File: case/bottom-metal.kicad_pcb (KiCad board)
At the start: 2 copper layers, 135 x 93.7 mm, 5 parts

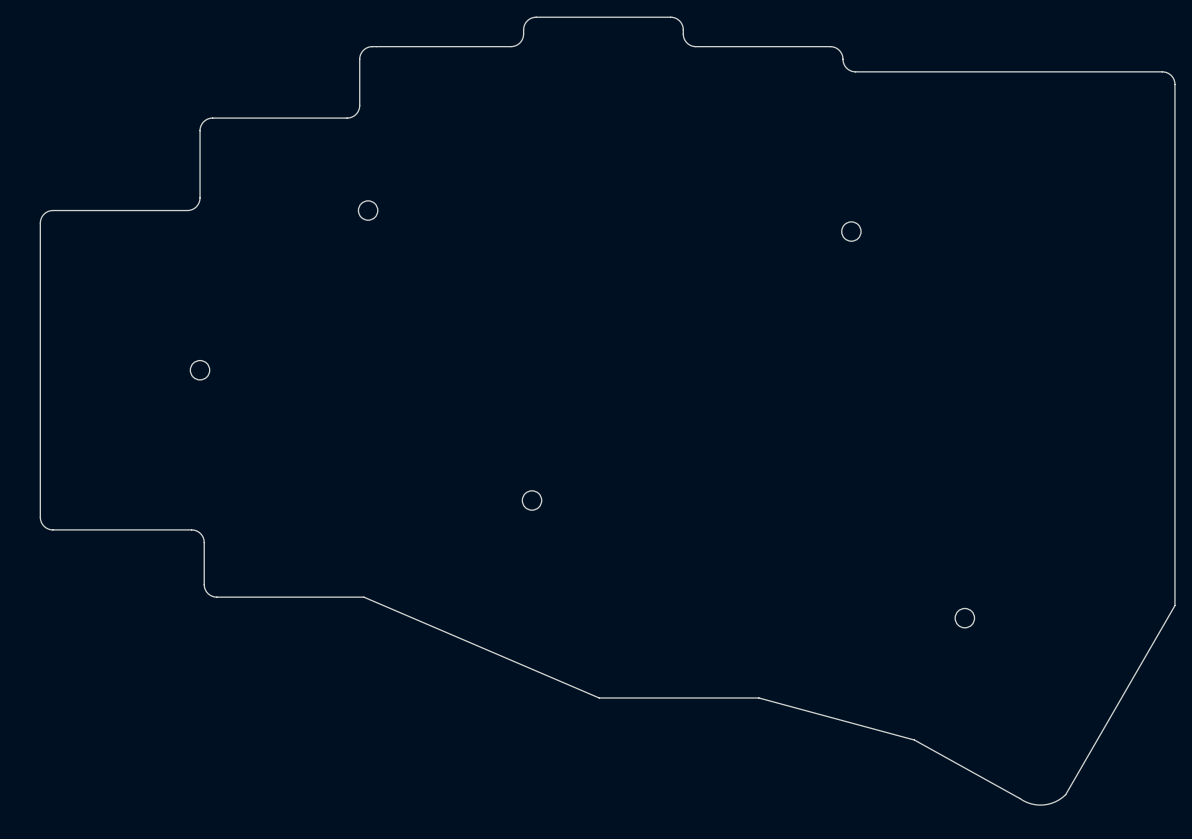
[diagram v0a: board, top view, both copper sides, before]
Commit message: update case files
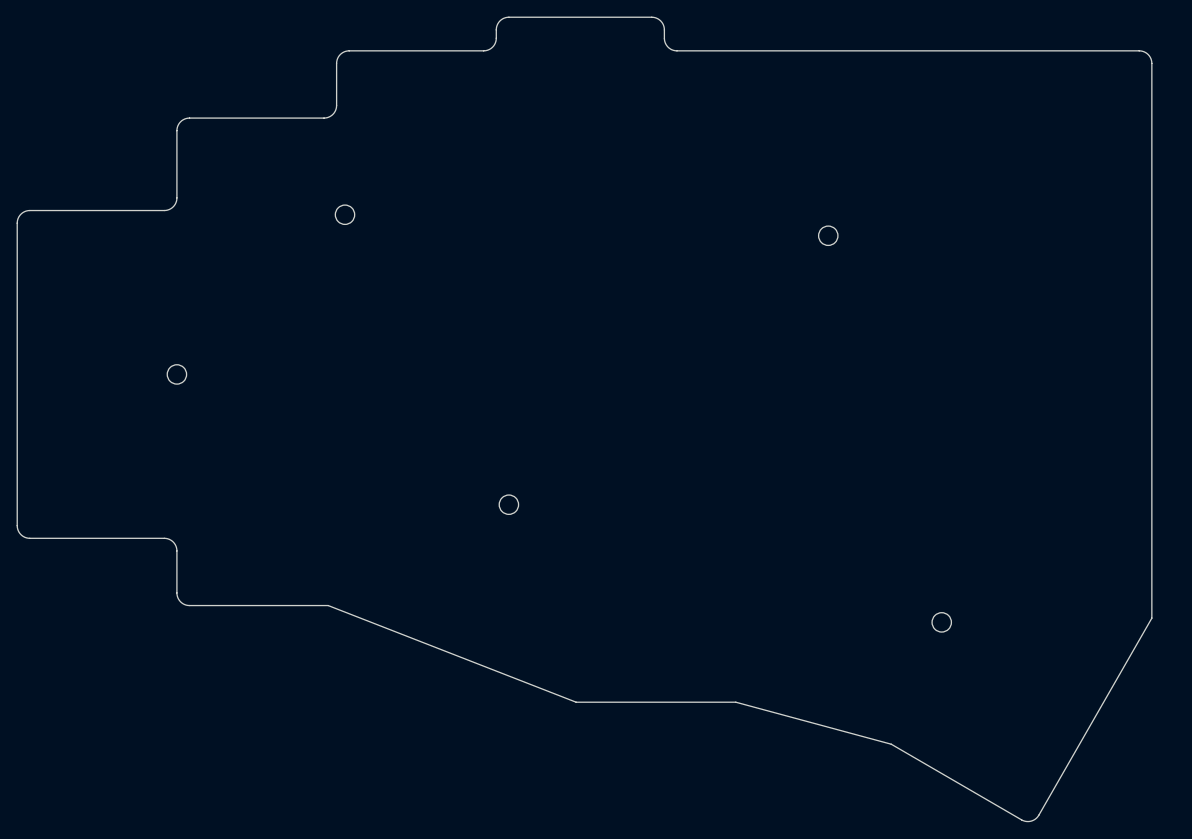
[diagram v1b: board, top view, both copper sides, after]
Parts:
- moved H1 2.80 mm to (104.8, 75.0)
- moved H2 2.80 mm to (175.8, 123.5)
- moved H3 2.80 mm to (84.8, 94.0)
- moved H4 2.80 mm to (124.2, 109.5)
- moved H5 2.80 mm to (162.2, 77.5)
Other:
- board size 135 x 93.7 mm -> 135 x 95.7 mm
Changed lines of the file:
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@@
       (drillshape 0)
       (scaleselection 1)
-      (outputdirectory "gerber/")
+      (outputdirectory "dxf/")
     )
   )
   (net 0 "")
   (footprint "kbd:thread_m2" (layer "F.Cu")
-    (at 178.5 123)
+    (at 175.75 123.5)
     (descr "Mounting Hole 2.2mm, no annular, M2")
     (tags "mounting hole 2.2mm no annular m2")
@@
   )
   (footprint "kbd:thread_m2" (layer "F.Cu")
-    (at 87.5 93.5)
+    (at 84.75 94)
     (descr "Mounting Hole 2.2mm, no annular, M2")
     (tags "mounting hole 2.2mm no annular m2")
@@
   )
   (footprint "kbd:thread_m2" (layer "F.Cu")
-    (at 165 77)
+    (at 124.25 109.5)
     (descr "Mounting Hole 2.2mm, no annular, M2")
     (tags "mounting hole 2.2mm no annular m2")
@@
     (property "Sheetname" "")
     (attr exclude_from_pos_files exclude_from_bom)
-    (fp_text reference "H5" (at -0.95 -0.55) (layer "F.Fab") hide
+    (fp_text reference "H4" (at -0.95 -0.55) (layer "F.Fab") hide
       (effects (font (size 1 1) (thickness 0.15)))
     )
@@
   )
   (footprint "kbd:thread_m2" (layer "F.Cu")
-    (at 107.5 74.5)
+    (at 104.75 75)
     (descr "Mounting Hole 2.2mm, no annular, M2")
     (tags "mounting hole 2.2mm no annular m2")
@@
   )
   (footprint "kbd:thread_m2" (layer "F.Cu")
-    (at 127 109)
+    (at 162.25 77.5)
     (descr "Mounting Hole 2.2mm, no annular, M2")
     (tags "mounting hole 2.2mm no annular m2")
@@
     (property "Sheetname" "")
     (attr exclude_from_pos_files exclude_from_bom)
-    (fp_text reference "H4" (at -0.95 -0.55) (layer "F.Fab") hide
+    (fp_text reference "H5" (at -0.95 -0.55) (layer "F.Fab") hide
       (effects (font (size 1 1) (thickness 0.15)))
     )
@@
     (pad "" np_thru_hole circle locked (at 0 0) (size 2.3 2.3) (drill 2.3) (layers *.Cu *.Mask))
   )
-  (gr_line (start 126 53) (end 126 53.5) (layer "Edge.Cuts") (width 0.1))
-  (gr_line (start 145 53.5) (end 145 53) (layer "Edge.Cuts") (width 0.1))
-  (gr_line (start 135 132.5) (end 154 132.5) (layer "Edge.Cuts") (width 0.1))
-  (gr_line (start 190.5 144) (end 203.5 121.5) (layer "Edge.Cuts") (width 0.1))
-  (gr_line (start 202 58) (end 165.5 58) (layer "Edge.Cuts") (width 0.1))
-  (gr_line (start 89.5 120.5) (end 107 120.5) (layer "Edge.Cuts") (width 0.1))
-  (gr_arc (start 86.5 112.5) (mid 87.56066 112.93934) (end 88 114) (layer "Edge.Cuts") (width 0.1))
-  (gr_line (start 87.5 65) (end 87.5 73) (layer "Edge.Cuts") (width 0.1))
-  (gr_arc (start 87.5 65) (mid 87.93934 63.93934) (end 89 63.5) (layer "Edge.Cuts") (width 0.1))
-  (gr_line (start 143.5 51.5) (end 127.5 51.5) (layer "Edge.Cuts") (width 0.1))
-  (gr_arc (start 106.5 62) (mid 106.06066 63.06066) (end 105 63.5) (layer "Edge.Cuts") (width 0.1))
-  (gr_line (start 107 120.5) (end 135 132.5) (layer "Edge.Cuts") (width 0.1))
-  (gr_arc (start 202 58) (mid 203.06066 58.43934) (end 203.5 59.5) (layer "Edge.Cuts") (width 0.1))
-  (gr_arc (start 68.5 76) (mid 68.93934 74.93934) (end 70 74.5) (layer "Edge.Cuts") (width 0.1))
-  (gr_line (start 203.5 121.5) (end 203.5 59.5) (layer "Edge.Cuts") (width 0.1))
-  (gr_line (start 108.5 55) (end 108 55) (layer "Edge.Cuts") (width 0.1))
-  (gr_arc (start 89.5 120.5) (mid 88.43934 120.06066) (end 88 119) (layer "Edge.Cuts") (width 0.1))
-  (gr_arc (start 165.5 58) (mid 164.43934 57.56066) (end 164 56.5) (layer "Edge.Cuts") (width 0.1))
-  (gr_arc (start 70 112.5) (mid 68.93934 112.06066) (end 68.5 111) (layer "Edge.Cuts") (width 0.1))
-  (gr_line (start 105 63.5) (end 89 63.5) (layer "Edge.Cuts") (width 0.1))
-  (gr_line (start 88 114) (end 88 119) (layer "Edge.Cuts") (width 0.1))
-  (gr_line (start 106.5 56.5) (end 106.5 62) (layer "Edge.Cuts") (width 0.1))
-  (gr_arc (start 190.5 144) (mid 187.849935 145.228185) (end 185.034016 144.452378) (layer "Edge.Cuts") (width 0.1))
-  (gr_line (start 124.5 55) (end 108.5 55) (layer "Edge.Cuts") (width 0.1))
-  (gr_arc (start 143.5 51.5) (mid 144.56066 51.93934) (end 145 53) (layer "Edge.Cuts") (width 0.1))
-  (gr_line (start 86 74.5) (end 70 74.5) (layer "Edge.Cuts") (width 0.1))
-  (gr_arc (start 87.5 73) (mid 87.06066 74.06066) (end 86 74.5) (layer "Edge.Cuts") (width 0.1))
-  (gr_arc (start 146.5 55) (mid 145.43934 54.56066) (end 145 53.5) (layer "Edge.Cuts") (width 0.1))
-  (gr_arc (start 126 53.5) (mid 125.56066 54.56066) (end 124.5 55) (layer "Edge.Cuts") (width 0.1))
-  (gr_arc (start 126 53) (mid 126.43934 51.93934) (end 127.5 51.5) (layer "Edge.Cuts") (width 0.1))
-  (gr_line (start 70 112.5) (end 86.5 112.5) (layer "Edge.Cuts") (width 0.1))
-  (gr_arc (start 162.5 55) (mid 163.56066 55.43934) (end 164 56.5) (layer "Edge.Cuts") (width 0.1))
-  (gr_line (start 185.034016 144.452378) (end 172.5 137.5) (layer "Edge.Cuts") (width 0.1))
-  (gr_line (start 162.5 55) (end 146.5 55) (layer "Edge.Cuts") (width 0.1))
-  (gr_arc (start 106.5 56.5) (mid 106.93934 55.43934) (end 108 55) (layer "Edge.Cuts") (width 0.1))
-  (gr_line (start 68.5 76) (end 68.5 111) (layer "Edge.Cuts") (width 0.1))
-  (gr_line (start 154 132.5) (end 172.5 137.5) (layer "Edge.Cuts") (width 0.1))
+  (gr_line (start 141.25 51.5) (end 124.25 51.5) (layer "Edge.Cuts") (width 0.1))
+  (gr_arc (start 84.75 65) (mid 85.18934 63.93934) (end 86.25 63.5) (layer "Edge.Cuts") (width 0.1))
+  (gr_arc (start 83.25 113.5) (mid 84.31066 113.93934) (end 84.75 115) (layer "Edge.Cuts") (width 0.1))
+  (gr_arc (start 144.25 55.5) (mid 143.18934 55.06066) (end 142.75 54) (layer "Edge.Cuts") (width 0.1))
+  (gr_line (start 86.25 121.5) (end 102.75 121.5) (layer "Edge.Cuts") (width 0.1))
+  (gr_line (start 103.75 57) (end 103.75 62) (layer "Edge.Cuts") (width 0.1))
+  (gr_arc (start 103.75 57) (mid 104.18934 55.93934) (end 105.25 55.5) (layer "Edge.Cuts") (width 0.1))
+  (gr_line (start 151.25 133) (end 169.75 138) (layer "Edge.Cuts") (width 0.1))
+  (gr_line (start 199.25 55.5) (end 144.25 55.5) (layer "Edge.Cuts") (width 0.1))
+  (gr_arc (start 199.25 55.5) (mid 200.31066 55.93934) (end 200.75 57) (layer "Edge.Cuts") (width 0.1))
+  (gr_arc (start 67.25 113.5) (mid 66.18934 113.06066) (end 65.75 112) (layer "Edge.Cuts") (width 0.1))
+  (gr_line (start 102.25 63.5) (end 86.25 63.5) (layer "Edge.Cuts") (width 0.1))
+  (gr_line (start 200.75 123) (end 200.75 57) (layer "Edge.Cuts") (width 0.1))
+  (gr_line (start 185.25 147) (end 169.75 138) (layer "Edge.Cuts") (width 0.1))
+  (gr_line (start 121.25 55.5) (end 105.25 55.5) (layer "Edge.Cuts") (width 0.1))
+  (gr_line (start 187.299038 146.450962) (end 200.75 123) (layer "Edge.Cuts") (width 0.1))
+  (gr_line (start 84.75 65) (end 84.75 73) (layer "Edge.Cuts") (width 0.1))
+  (gr_line (start 132.25 133) (end 151.25 133) (layer "Edge.Cuts") (width 0.1))
+  (gr_arc (start 84.75 73) (mid 84.31066 74.06066) (end 83.25 74.5) (layer "Edge.Cuts") (width 0.1))
+  (gr_line (start 67.25 113.5) (end 83.25 113.5) (layer "Edge.Cuts") (width 0.1))
+  (gr_arc (start 86.25 121.5) (mid 85.18934 121.06066) (end 84.75 120) (layer "Edge.Cuts") (width 0.1))
+  (gr_arc (start 141.25 51.5) (mid 142.31066 51.93934) (end 142.75 53) (layer "Edge.Cuts") (width 0.1))
+  (gr_arc (start 187.299038 146.450962) (mid 186.388233 147.149868) (end 185.25 147) (layer "Edge.Cuts") (width 0.1))
+  (gr_line (start 122.75 53) (end 122.75 54) (layer "Edge.Cuts") (width 0.1))
+  (gr_line (start 83.25 74.5) (end 67.25 74.5) (layer "Edge.Cuts") (width 0.1))
+  (gr_line (start 65.75 76) (end 65.75 112) (layer "Edge.Cuts") (width 0.1))
+  (gr_arc (start 103.75 62) (mid 103.31066 63.06066) (end 102.25 63.5) (layer "Edge.Cuts") (width 0.1))
+  (gr_line (start 102.75 121.5) (end 132.25 133) (layer "Edge.Cuts") (width 0.1))
+  (gr_arc (start 122.75 53) (mid 123.18934 51.93934) (end 124.25 51.5) (layer "Edge.Cuts") (width 0.1))
+  (gr_line (start 84.75 115) (end 84.75 120) (layer "Edge.Cuts") (width 0.1))
+  (gr_line (start 142.75 54) (end 142.75 53) (layer "Edge.Cuts") (width 0.1))
+  (gr_arc (start 122.75 54) (mid 122.31066 55.06066) (end 121.25 55.5) (layer "Edge.Cuts") (width 0.1))
+  (gr_arc (start 65.75 76) (mid 66.18934 74.93934) (end 67.25 74.5) (layer "Edge.Cuts") (width 0.1))
 )
